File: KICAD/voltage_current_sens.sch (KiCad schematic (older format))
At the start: 17 parts

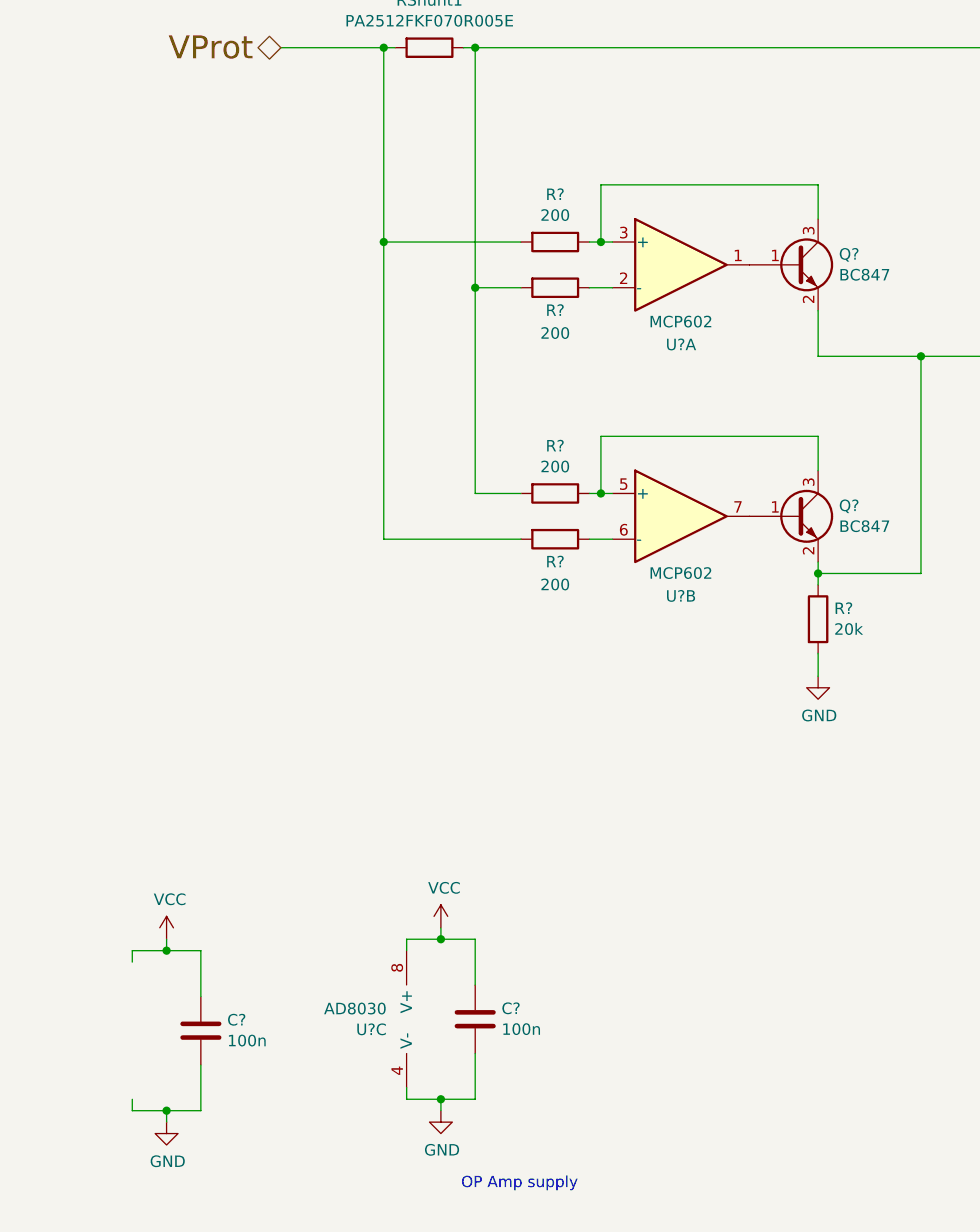
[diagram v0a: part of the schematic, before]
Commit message: lt6015 it is
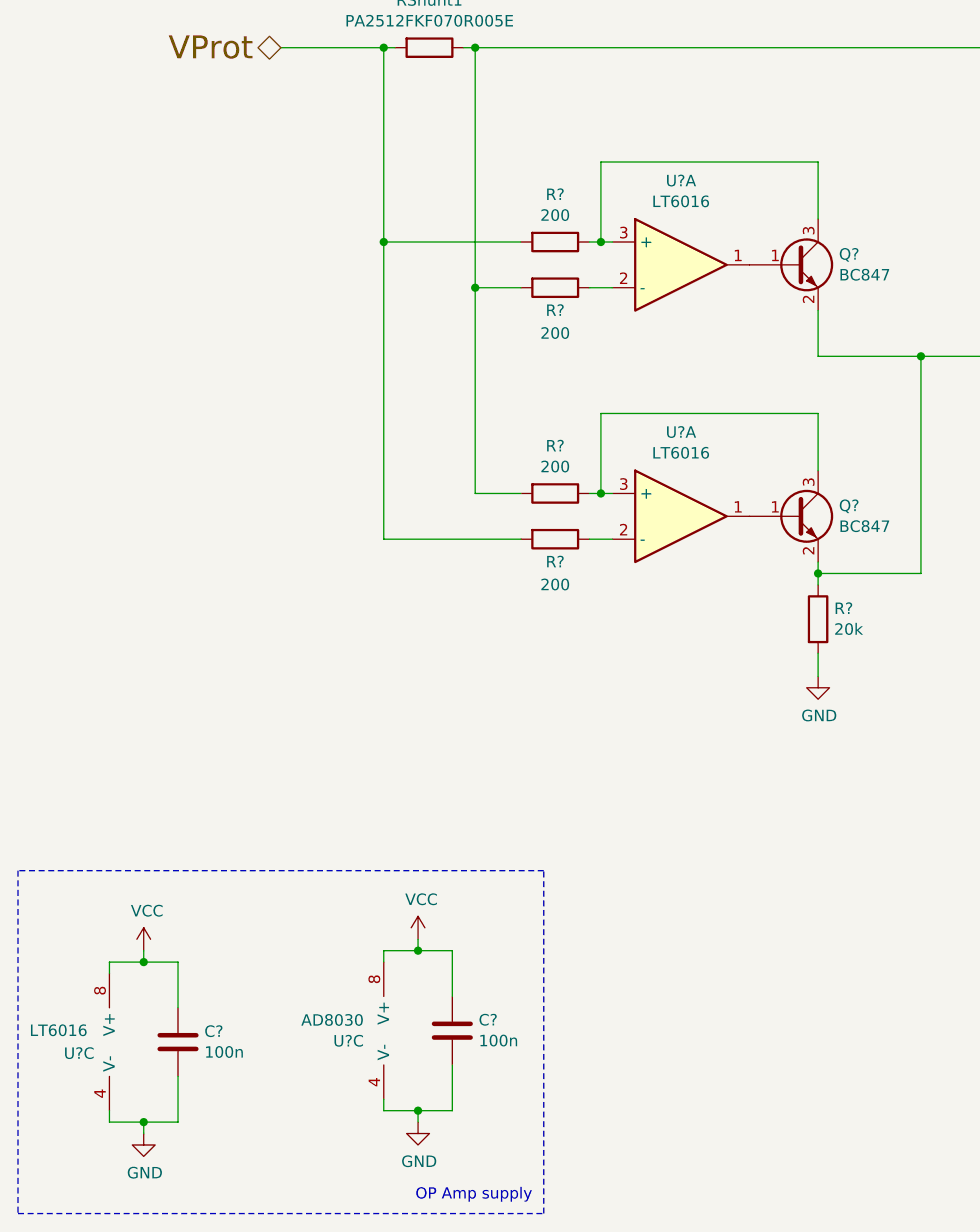
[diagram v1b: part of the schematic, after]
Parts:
- removed U? (x2): MCP602, symbol Amplifier_Operational:MCP602
- added U? (x3): LT6016, Package_SO:MSOP-8_3x3mm_P0.65mm, symbol Sesame:LT6016
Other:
- moved on the sheet: C?, U?C
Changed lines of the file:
@@
 	9000 3250 8700 3250
 Connection ~ 8700 3250
-$Comp
-L Amplifier_Operational:MCP602 U?
-U 2 1 614506A4
-P 3450 4650
-AR Path="/60F19D5B/614506A4" Ref="U?"  Part="1"
-AR Path="/60F171CE/614506A4" Ref="U?"  Part="2"
-F 0 "U?" H 3450 4300 50  0000 C CNN
-F 1 "MCP602" H 3450 4400 50  0000 C CNN
-F 2 "" H 3450 4650 50  0001 C CNN
-F 3 "http://ww1.microchip.com/downloads/en/DeviceDoc/21314g.pdf" H 3450 4650 50  0001 C CNN
-	2    3450 4650
-	1    0    0    -1
-$EndComp
 Wire Wire Line
 	2550 4550 2750 4550
@@
 Wire Wire Line
 	2150 2600 2150 3450
-$Comp
-L Amplifier_Operational:MCP602 U?
-U 1 1 61378B89
-P 3450 3550
-AR Path="/60F19D5B/61378B89" Ref="U?"  Part="1"
-AR Path="/60F171CE/61378B89" Ref="U?"  Part="1"
-F 0 "U?" H 3450 3200 50  0000 C CNN
-F 1 "MCP602" H 3450 3300 50  0000 C CNN
-F 2 "" H 3450 3550 50  0001 C CNN
-F 3 "http://ww1.microchip.com/downloads/en/DeviceDoc/21314g.pdf" H 3450 3550 50  0001 C CNN
-	1    3450 3550
-	1    0    0    -1
-$EndComp
 Wire Wire Line
 	2750 3450 2150 3450
@@
 	1    0    0    -1
 $EndComp
-Wire Wire Line
-	3100 3200 4050 3200
-Wire Wire Line
-	4050 3200 4050 3350
-Wire Wire Line
-	3100 3200 3100 3450
 Connection ~ 3100 3450
 Wire Wire Line
 	3100 3450 3150 3450
-Wire Wire Line
-	3100 4550 3100 4300
-Wire Wire Line
-	3100 4300 4050 4300
-Wire Wire Line
-	4050 4300 4050 4450
 Connection ~ 3100 4550
 Wire Wire Line
@@
 L Device:C C?
 U 1 1 613B4715
-P 1350 6900
+P 1250 6950
 AR Path="/60F1AF26/613B4715" Ref="C?"  Part="1"
 AR Path="/60F1B237/613B4715" Ref="C?"  Part="1"
@@
 AR Path="/60F171CE/613B4715" Ref="C?"  Part="1"
 AR Path="/60F19D5B/613B4715" Ref="C?"  Part="1"
-F 0 "C?" H 1465 6946 50  0000 L CNN
-F 1 "100n" H 1465 6855 50  0000 L CNN
-F 2 "" H 1388 6750 50  0001 C CNN
-F 3 "~" H 1350 6900 50  0001 C CNN
-	1    1350 6900
-	1    0    0    -1
-$EndComp
-Wire Wire Line
-	1200 6500 1200 6550
-Wire Wire Line
-	1200 6550 1050 6550
-Wire Wire Line
-	1050 6550 1050 6600
-Connection ~ 1200 6550
-Wire Wire Line
-	1050 7250 1050 7200
+F 0 "C?" H 1365 6996 50  0000 L CNN
+F 1 "100n" H 1365 6905 50  0000 L CNN
+F 2 "" H 1288 6800 50  0001 C CNN
+F 3 "~" H 1250 6950 50  0001 C CNN
+	1    1250 6950
+	1    0    0    -1
+$EndComp
+Wire Wire Line
+	1100 6550 1100 6600
+Wire Wire Line
+	1100 6600 950  6600
+Wire Wire Line
+	950  6600 950  6650
+Connection ~ 1100 6600
+Wire Wire Line
+	950  7300 950  7250
 $Comp
 L power:GND #PWR?
 U 1 1 613B4720
-P 1200 7300
+P 1100 7350
 AR Path="/60F1AF26/613B4720" Ref="#PWR?"  Part="1"
 AR Path="/60F1B237/613B4720" Ref="#PWR?"  Part="1"
@@
 AR Path="/60F171CE/613B4720" Ref="#PWR?"  Part="1"
 AR Path="/60F19D5B/613B4720" Ref="#PWR?"  Part="1"
-F 0 "#PWR?" H 1200 7050 50  0001 C CNN
-F 1 "GND" H 1205 7127 50  0000 C CNN
-F 2 "" H 1200 7300 50  0001 C CNN
-F 3 "" H 1200 7300 50  0001 C CNN
-	1    1200 7300
-	1    0    0    -1
-$EndComp
-Wire Wire Line
-	1200 7300 1200 7250
-Connection ~ 1200 7250
-Wire Wire Line
-	1200 7250 1050 7250
-Wire Wire Line
-	1350 6550 1350 6750
-Wire Wire Line
-	1200 6550 1350 6550
-Wire Wire Line
-	1350 7050 1350 7250
-Wire Wire Line
-	1200 7250 1350 7250
+F 0 "#PWR?" H 1100 7100 50  0001 C CNN
+F 1 "GND" H 1105 7177 50  0000 C CNN
+F 2 "" H 1100 7350 50  0001 C CNN
+F 3 "" H 1100 7350 50  0001 C CNN
+	1    1100 7350
+	1    0    0    -1
+$EndComp
+Wire Wire Line
+	1100 7350 1100 7300
+Connection ~ 1100 7300
+Wire Wire Line
+	1100 7300 950  7300
+Wire Wire Line
+	1250 6600 1250 6800
+Wire Wire Line
+	1100 6600 1250 6600
+Wire Wire Line
+	1250 7100 1250 7300
+Wire Wire Line
+	1100 7300 1250 7300
 $Comp
 L power:VCC #PWR?
 U 1 1 613B472D
-P 1200 6500
+P 1100 6550
 AR Path="/60F1AF26/613B472D" Ref="#PWR?"  Part="1"
 AR Path="/60F1B237/613B472D" Ref="#PWR?"  Part="1"
@@
 AR Path="/60F171CE/613B472D" Ref="#PWR?"  Part="1"
 AR Path="/60F19D5B/613B472D" Ref="#PWR?"  Part="1"
-F 0 "#PWR?" H 1200 6350 50  0001 C CNN
-F 1 "VCC" H 1215 6673 50  0000 C CNN
-F 2 "" H 1200 6500 50  0001 C CNN
-F 3 "" H 1200 6500 50  0001 C CNN
-	1    1200 6500
-	1    0    0    -1
-$EndComp
-Text Notes 3000 7600 2    49   ~ 0
+F 0 "#PWR?" H 1100 6400 50  0001 C CNN
+F 1 "VCC" H 1115 6723 50  0000 C CNN
+F 2 "" H 1100 6550 50  0001 C CNN
+F 3 "" H 1100 6550 50  0001 C CNN
+	1    1100 6550
+	1    0    0    -1
+$EndComp
+Text Notes 2800 7650 2    49   ~ 0
 OP Amp supply
 $Comp
 L Device:C C?
 U 1 1 613B7585
-P 2550 6850
+P 2450 6900
 AR Path="/60F1AF26/613B7585" Ref="C?"  Part="1"
 AR Path="/60F1B237/613B7585" Ref="C?"  Part="1"
@@
 AR Path="/60F171CE/613B7585" Ref="C?"  Part="1"
 AR Path="/60F19D5B/613B7585" Ref="C?"  Part="1"
-F 0 "C?" H 2665 6896 50  0000 L CNN
-F 1 "100n" H 2665 6805 50  0000 L CNN
-F 2 "" H 2588 6700 50  0001 C CNN
-F 3 "~" H 2550 6850 50  0001 C CNN
-	1    2550 6850
-	1    0    0    -1
-$EndComp
-Wire Wire Line
-	2400 6450 2400 6500
-Wire Wire Line
-	2400 6500 2250 6500
-Wire Wire Line
-	2250 6500 2250 6550
-Connection ~ 2400 6500
-Wire Wire Line
-	2250 7200 2250 7150
+F 0 "C?" H 2565 6946 50  0000 L CNN
+F 1 "100n" H 2565 6855 50  0000 L CNN
+F 2 "" H 2488 6750 50  0001 C CNN
+F 3 "~" H 2450 6900 50  0001 C CNN
+	1    2450 6900
+	1    0    0    -1
+$EndComp
+Wire Wire Line
+	2300 6500 2300 6550
+Wire Wire Line
+	2300 6550 2150 6550
+Wire Wire Line
+	2150 6550 2150 6600
+Connection ~ 2300 6550
+Wire Wire Line
+	2150 7250 2150 7200
 $Comp
 L power:GND #PWR?
 U 1 1 613B7590
-P 2400 7250
+P 2300 7300
 AR Path="/60F1AF26/613B7590" Ref="#PWR?"  Part="1"
 AR Path="/60F1B237/613B7590" Ref="#PWR?"  Part="1"
@@
 AR Path="/60F171CE/613B7590" Ref="#PWR?"  Part="1"
 AR Path="/60F19D5B/613B7590" Ref="#PWR?"  Part="1"
-F 0 "#PWR?" H 2400 7000 50  0001 C CNN
-F 1 "GND" H 2405 7077 50  0000 C CNN
-F 2 "" H 2400 7250 50  0001 C CNN
-F 3 "" H 2400 7250 50  0001 C CNN
-	1    2400 7250
-	1    0    0    -1
-$EndComp
-Wire Wire Line
-	2400 7250 2400 7200
-Connection ~ 2400 7200
-Wire Wire Line
-	2400 7200 2250 7200
-Wire Wire Line
-	2550 6500 2550 6700
-Wire Wire Line
-	2400 6500 2550 6500
-Wire Wire Line
-	2550 7000 2550 7200
-Wire Wire Line
-	2400 7200 2550 7200
+F 0 "#PWR?" H 2300 7050 50  0001 C CNN
+F 1 "GND" H 2305 7127 50  0000 C CNN
+F 2 "" H 2300 7300 50  0001 C CNN
+F 3 "" H 2300 7300 50  0001 C CNN
+	1    2300 7300
+	1    0    0    -1
+$EndComp
+Wire Wire Line
+	2300 7300 2300 7250
+Connection ~ 2300 7250
+Wire Wire Line
+	2300 7250 2150 7250
+Wire Wire Line
+	2450 6550 2450 6750
+Wire Wire Line
+	2300 6550 2450 6550
+Wire Wire Line
+	2450 7050 2450 7250
+Wire Wire Line
+	2300 7250 2450 7250
 $Comp
 L power:VCC #PWR?
 U 1 1 613B759D
-P 2400 6450
+P 2300 6500
 AR Path="/60F1AF26/613B759D" Ref="#PWR?"  Part="1"
 AR Path="/60F1B237/613B759D" Ref="#PWR?"  Part="1"
@@
 AR Path="/60F171CE/613B759D" Ref="#PWR?"  Part="1"
 AR Path="/60F19D5B/613B759D" Ref="#PWR?"  Part="1"
-F 0 "#PWR?" H 2400 6300 50  0001 C CNN
-F 1 "VCC" H 2415 6623 50  0000 C CNN
-F 2 "" H 2400 6450 50  0001 C CNN
-F 3 "" H 2400 6450 50  0001 C CNN
-	1    2400 6450
+F 0 "#PWR?" H 2300 6350 50  0001 C CNN
+F 1 "VCC" H 2315 6673 50  0000 C CNN
+F 2 "" H 2300 6500 50  0001 C CNN
+F 3 "" H 2300 6500 50  0001 C CNN
+	1    2300 6500
 	1    0    0    -1
 $EndComp
@@
 L Sesame:AD8030 U?
 U 3 1 613B75A3
-P 2350 6850
+P 2250 6900
 AR Path="/60F1AF26/613B75A3" Ref="U?"  Part="3"
 AR Path="/60F1B237/613B75A3" Ref="U?"  Part="3"
@@
 AR Path="/60F171CE/613B75A3" Ref="U?"  Part="3"
 AR Path="/60F19D5B/613B75A3" Ref="U?"  Part="3"
-F 0 "U?" H 2163 6804 50  0000 R CNN
-F 1 "AD8030" H 2163 6895 50  0000 R CNN
-F 2 "" H 2350 6850 50  0001 C CNN
-F 3 "~" H 2350 6850 50  0001 C CNN
-	3    2350 6850
-	1    0    0    -1
-$EndComp
+F 0 "U?" H 2063 6854 50  0000 R CNN
+F 1 "AD8030" H 2063 6945 50  0000 R CNN
+F 2 "" H 2250 6900 50  0001 C CNN
+F 3 "~" H 2250 6900 50  0001 C CNN
+	3    2250 6900
+	1    0    0    -1
+$EndComp
+$Comp
+L Sesame:LT6016 U?
+U 1 1 615B8C9F
+P 3450 3550
+F 0 "U?" H 3450 3917 50  0000 C CNN
+F 1 "LT6016" H 3450 3826 50  0000 C CNN
+F 2 "Package_SO:MSOP-8_3x3mm_P0.65mm" H 3450 3550 50  0001 C CNN
+F 3 "~" H 3450 3550 50  0001 C CNN
+	1    3450 3550
+	1    0    0    -1
+$EndComp
+Wire Wire Line
+	4050 3100 3100 3100
+Wire Wire Line
+	3100 3100 3100 3450
+Wire Wire Line
+	4050 3100 4050 3350
+$Comp
+L Sesame:LT6016 U?
+U 1 1 615BC62A
+P 3450 4650
+F 0 "U?" H 3450 5017 50  0000 C CNN
+F 1 "LT6016" H 3450 4926 50  0000 C CNN
+F 2 "Package_SO:MSOP-8_3x3mm_P0.65mm" H 3450 4650 50  0001 C CNN
+F 3 "~" H 3450 4650 50  0001 C CNN
+	1    3450 4650
+	1    0    0    -1
+$EndComp
+Wire Wire Line
+	3100 4200 4050 4200
+Wire Wire Line
+	3100 4200 3100 4550
+Wire Wire Line
+	4050 4200 4050 4450
+$Comp
+L Sesame:LT6016 U?
+U 3 1 615BFCFC
+P 1050 6950
+F 0 "U?" H 750 6900 50  0000 L CNN
+F 1 "LT6016" H 600 7000 50  0000 L CNN
+F 2 "Package_SO:MSOP-8_3x3mm_P0.65mm" H 1050 6950 50  0001 C CNN
+F 3 "~" H 1050 6950 50  0001 C CNN
+	3    1050 6950
+	1    0    0    -1
+$EndComp
+Wire Notes Line
+	550  7700 2850 7700
+Wire Notes Line
+	2850 7700 2850 6200
+Wire Notes Line
+	2850 6200 550  6200
+Wire Notes Line
+	550  6200 550  7700
 $EndSCHEMATC

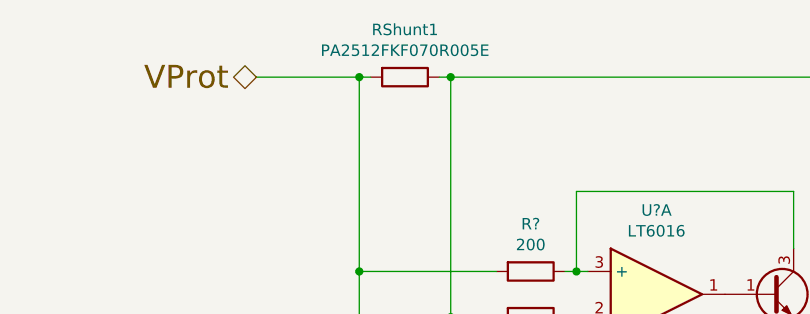
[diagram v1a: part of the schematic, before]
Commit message: mainly footprints
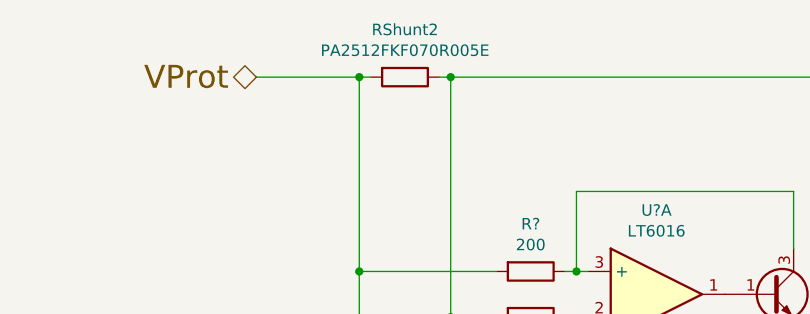
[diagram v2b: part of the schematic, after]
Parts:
- R? (x7): footprint (none) -> Resistor_SMD:R_0805_2012Metric_Pad1.15x1.40mm_HandSolder
- U? (x3): footprint (none) -> Package_SO:SO-8_3.9x4.9mm_P1.27mm
- renumbered RShunt1 to RShunt2
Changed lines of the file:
@@
 $Descr A4 11693 8268
 encoding utf-8
-Sheet 10 16
+Sheet 13 16
 Title "SESAME"
 Date ""
@@
 	2150 2600 1700 2600
 $Comp
-L Device:R RShunt1
+L Device:R RShunt2
 U 1 1 6109114F
 P 2350 2600
-AR Path="/60F19D5B/6109114F" Ref="RShunt1"  Part="1"
-AR Path="/60F171CE/6109114F" Ref="R?"  Part="1"
-F 0 "R?" V 2143 2600 50  0000 C CNN
+AR Path="/60F19D5B/6109114F" Ref="RShunt2"  Part="1"
+AR Path="/60F171CE/6109114F" Ref="RShunt1"  Part="1"
+F 0 "RShunt2" V 2143 2600 50  0000 C CNN
 F 1 "PA2512FKF070R005E" V 2234 2600 50  0000 C CNN
 F 2 "Resistor_SMD:R_2512_6332Metric_Pad1.40x3.35mm_HandSolder" V 2280 2600 50  0001 C CNN
@@
 F 0 "R?" V 3000 3650 50  0000 C CNN
 F 1 "200" V 3100 3650 50  0000 C CNN
-F 2 "" V 2830 3650 50  0001 C CNN
+F 2 "Resistor_SMD:R_0805_2012Metric_Pad1.15x1.40mm_HandSolder" V 2830 3650 50  0001 C CNN
 F 3 "~" H 2900 3650 50  0001 C CNN
 	1    2900 3650
@@
 F 0 "R?" V 2693 3450 50  0000 C CNN
 F 1 "200" V 2784 3450 50  0000 C CNN
-F 2 "" V 2830 3450 50  0001 C CNN
+F 2 "Resistor_SMD:R_0805_2012Metric_Pad1.15x1.40mm_HandSolder" V 2830 3450 50  0001 C CNN
 F 3 "~" H 2900 3450 50  0001 C CNN
 	1    2900 3450
@@
 AR Path="/60F171CE/610DEA27" Ref="#PWR0157"  Part="1"
 AR Path="/60F19D5B/610DEA27" Ref="#PWR0112"  Part="1"
-F 0 "#PWR0157" H 7650 3650 50  0001 C CNN
+F 0 "#PWR0112" H 7650 3650 50  0001 C CNN
 F 1 "GND" H 7655 3727 50  0000 C CNN
 F 2 "" H 7650 3900 50  0001 C CNN
@@
 F 0 "R?" H 7720 3746 50  0000 L CNN
 F 1 "10k" H 7720 3655 50  0000 L CNN
-F 2 "" V 7580 3700 50  0001 C CNN
+F 2 "Resistor_SMD:R_0805_2012Metric_Pad1.15x1.40mm_HandSolder" V 7580 3700 50  0001 C CNN
 F 3 "~" H 7650 3700 50  0001 C CNN
 	1    7650 3700
@@
 F 0 "R?" H 7720 3046 50  0000 L CNN
 F 1 "90k" H 7720 2955 50  0000 L CNN
-F 2 "" V 7580 3000 50  0001 C CNN
+F 2 "Resistor_SMD:R_0805_2012Metric_Pad1.15x1.40mm_HandSolder" V 7580 3000 50  0001 C CNN
 F 3 "~" H 7650 3000 50  0001 C CNN
 	1    7650 3000
@@
 F 0 "R?" H 4120 5146 50  0000 L CNN
 F 1 "20k" H 4120 5055 50  0000 L CNN
-F 2 "" V 3980 5100 50  0001 C CNN
+F 2 "Resistor_SMD:R_0805_2012Metric_Pad1.15x1.40mm_HandSolder" V 3980 5100 50  0001 C CNN
 F 3 "~" H 4050 5100 50  0001 C CNN
 	1    4050 5100
@@
 F 0 "R?" V 2693 4550 50  0000 C CNN
 F 1 "200" V 2784 4550 50  0000 C CNN
-F 2 "" V 2830 4550 50  0001 C CNN
+F 2 "Resistor_SMD:R_0805_2012Metric_Pad1.15x1.40mm_HandSolder" V 2830 4550 50  0001 C CNN
 F 3 "~" H 2900 4550 50  0001 C CNN
 	1    2900 4550
@@
 F 0 "R?" V 3000 4750 50  0000 C CNN
 F 1 "200" V 3100 4750 50  0000 C CNN
-F 2 "" V 2830 4750 50  0001 C CNN
+F 2 "Resistor_SMD:R_0805_2012Metric_Pad1.15x1.40mm_HandSolder" V 2830 4750 50  0001 C CNN
 F 3 "~" H 2900 4750 50  0001 C CNN
 	1    2900 4750
@@
 F 0 "U?" H 8350 2800 50  0000 C CNN
 F 1 "AD8030" H 8350 2900 50  0000 C CNN
-F 2 "" H 8350 3250 50  0001 C CNN
+F 2 "Package_SO:SO-8_3.9x4.9mm_P1.27mm" H 8350 3250 50  0001 C CNN
 F 3 "~" H 8350 3250 50  0001 C CNN
 	2    8350 3250
@@
 F 0 "U?" H 5200 3400 50  0000 C CNN
 F 1 "AD8030" H 5200 3500 50  0000 C CNN
-F 2 "" H 5200 3850 50  0001 C CNN
+F 2 "Package_SO:SO-8_3.9x4.9mm_P1.27mm" H 5200 3850 50  0001 C CNN
 F 3 "~" H 5200 3850 50  0001 C CNN
 	1    5200 3850
@@
 F 0 "U?" H 2063 6854 50  0000 R CNN
 F 1 "AD8030" H 2063 6945 50  0000 R CNN
-F 2 "" H 2250 6900 50  0001 C CNN
+F 2 "Package_SO:SO-8_3.9x4.9mm_P1.27mm" H 2250 6900 50  0001 C CNN
 F 3 "~" H 2250 6900 50  0001 C CNN
 	3    2250 6900
@@
 U 1 1 615B8C9F
 P 3450 3550
+AR Path="/60F171CE/615B8C9F" Ref="U?"  Part="1"
+AR Path="/60F19D5B/615B8C9F" Ref="U?"  Part="1"
 F 0 "U?" H 3450 3917 50  0000 C CNN
 F 1 "LT6016" H 3450 3826 50  0000 C CNN
@@
 U 1 1 615BC62A
 P 3450 4650
+AR Path="/60F171CE/615BC62A" Ref="U?"  Part="1"
+AR Path="/60F19D5B/615BC62A" Ref="U?"  Part="1"
 F 0 "U?" H 3450 5017 50  0000 C CNN
 F 1 "LT6016" H 3450 4926 50  0000 C CNN
@@
 U 3 1 615BFCFC
 P 1050 6950
+AR Path="/60F171CE/615BFCFC" Ref="U?"  Part="3"
+AR Path="/60F19D5B/615BFCFC" Ref="U?"  Part="3"
 F 0 "U?" H 750 6900 50  0000 L CNN
 F 1 "LT6016" H 600 7000 50  0000 L CNN
@@
 $EndComp
 Wire Notes Line
+	2850 7700 2850 6200
+Wire Notes Line
+	2850 6200 550  6200
+Wire Notes Line
+	550  6200 550  7700
+Wire Notes Line
 	550  7700 2850 7700
-Wire Notes Line
-	2850 7700 2850 6200
-Wire Notes Line
-	2850 6200 550  6200
-Wire Notes Line
-	550  6200 550  7700
 $EndSCHEMATC

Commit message: revex with jmt
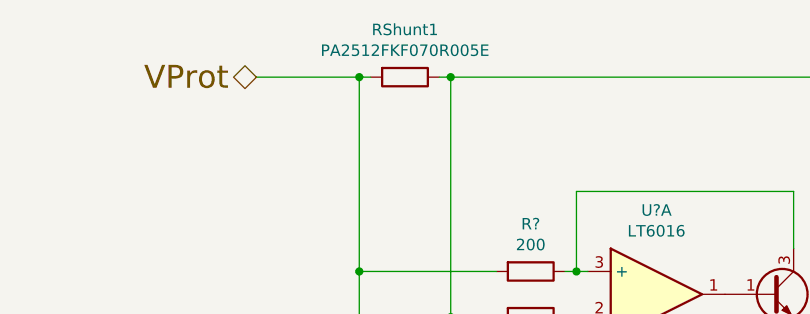
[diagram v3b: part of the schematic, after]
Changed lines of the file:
@@
 $Descr A4 11693 8268
 encoding utf-8
-Sheet 13 16
+Sheet 9 16
 Title "SESAME"
 Date ""
@@
 AR Path="/60F19D5B/6109114F" Ref="RShunt2"  Part="1"
 AR Path="/60F171CE/6109114F" Ref="RShunt1"  Part="1"
-F 0 "RShunt2" V 2143 2600 50  0000 C CNN
+F 0 "RShunt1" V 2143 2600 50  0000 C CNN
 F 1 "PA2512FKF070R005E" V 2234 2600 50  0000 C CNN
 F 2 "Resistor_SMD:R_2512_6332Metric_Pad1.40x3.35mm_HandSolder" V 2280 2600 50  0001 C CNN
@@
 AR Path="/60F171CE/610DEA27" Ref="#PWR0157"  Part="1"
 AR Path="/60F19D5B/610DEA27" Ref="#PWR0112"  Part="1"
-F 0 "#PWR0112" H 7650 3650 50  0001 C CNN
+F 0 "#PWR0157" H 7650 3650 50  0001 C CNN
 F 1 "GND" H 7655 3727 50  0000 C CNN
 F 2 "" H 7650 3900 50  0001 C CNN
